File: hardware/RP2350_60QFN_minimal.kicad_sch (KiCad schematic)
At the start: 37 parts, among them J4 SM03B-SRSS-TB, J5 4677, SW1 SW_Push, SW2 SW_Push, U1 RP2350_60QFN, U3 W25Q128JVS, Y1 ABM8-272-T3

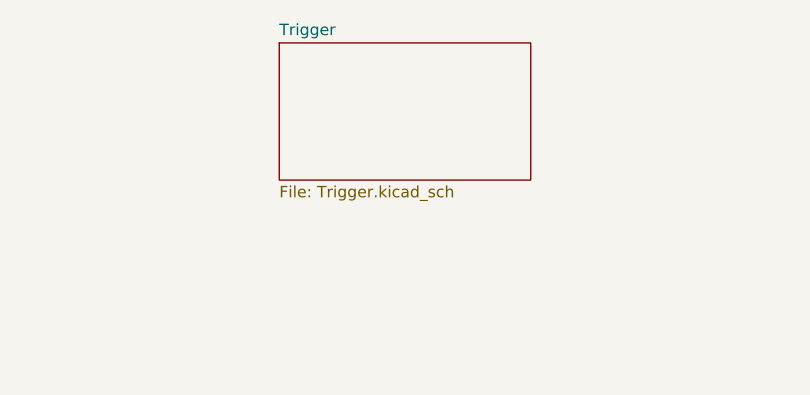
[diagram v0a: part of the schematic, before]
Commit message: Trig finished
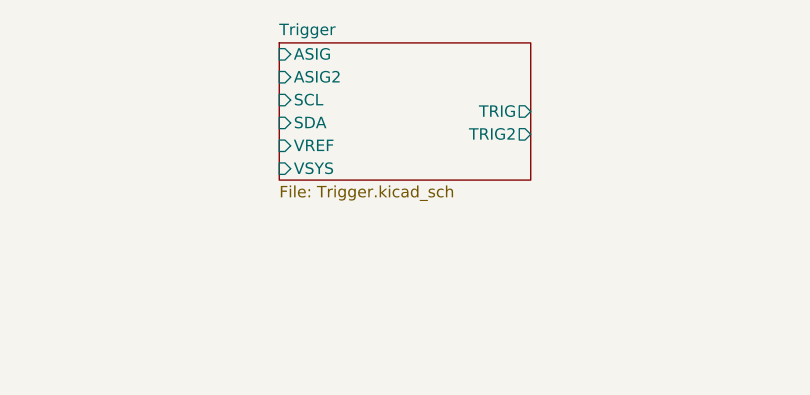
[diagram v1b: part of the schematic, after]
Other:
- sheet Trigger ports: added ASIG, ASIG2, SCL, SDA, TRIG, TRIG2, VREF, VSYS; removed none
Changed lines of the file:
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@@
+			)
+		)
+		(pin "ASIG" input
+			(at 189.23 45.72 180)
+			(effects
+				(font
+					(size 1.27 1.27)
+				)
+				(justify left)
+			)
+		)
+		(pin "ASIG2" input
+			(at 189.23 48.26 180)
+			(effects
+				(font
+					(size 1.27 1.27)
+				)
+				(justify left)
+			)
+		)
+		(pin "SCL" input
+			(at 189.23 50.8 180)
+			(effects
+				(font
+					(size 1.27 1.27)
+				)
+				(justify left)
+			)
+		)
+		(pin "SDA" input
+			(at 189.23 53.34 180)
+			(effects
+				(font
+					(size 1.27 1.27)
+				)
+				(justify left)
+			)
+		)
+		(pin "TRIG" output
+			(at 217.17 52.07 0)
+			(effects
+				(font
+					(size 1.27 1.27)
+				)
+				(justify right)
+			)
+		)
+		(pin "VREF" input
+			(at 189.23 55.88 180)
+			(effects
+				(font
+					(size 1.27 1.27)
+				)
+				(justify left)
+			)
+		)
+		(pin "VSYS" input
+			(at 189.23 58.42 180)
+			(effects
+				(font
+					(size 1.27 1.27)
+				)
+				(justify left)
+			)
+		)
+		(pin "TRIG2" output
+			(at 217.17 54.61 0)
+			(effects
+				(font
+					(size 1.27 1.27)
+				)
+				(justify right)
 			)
 		)
